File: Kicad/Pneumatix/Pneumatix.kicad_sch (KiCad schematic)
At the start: 22 parts, among them J1 Conn_01x06_Socket, J2 436500404, J3 142-0701-801, U1 E22-400T33S

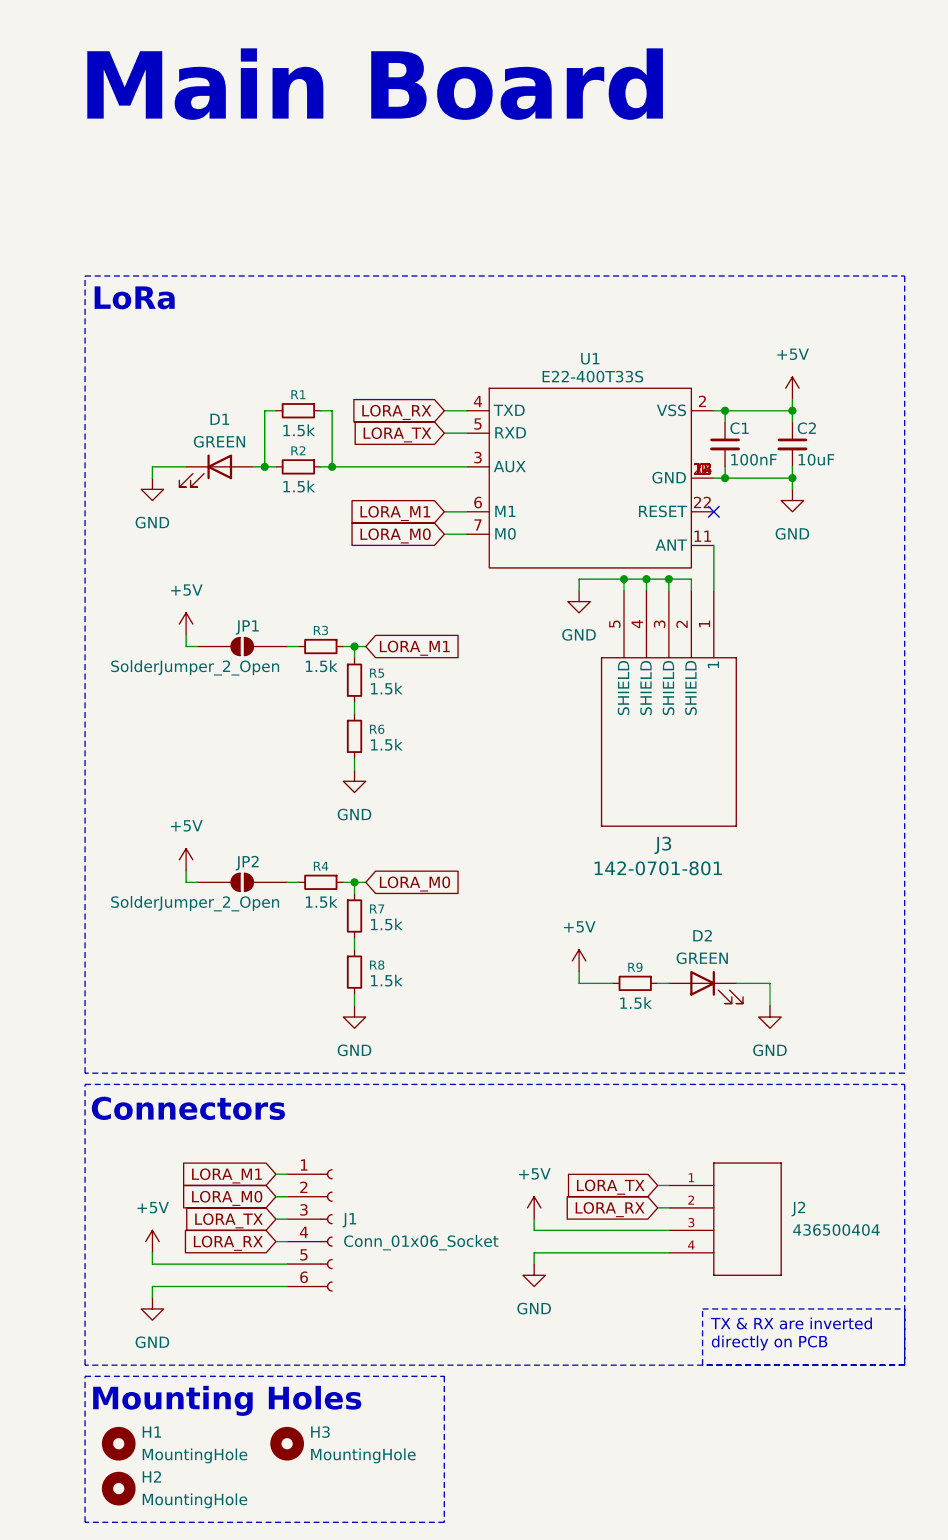
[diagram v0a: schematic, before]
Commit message: wip: pcb adjustements
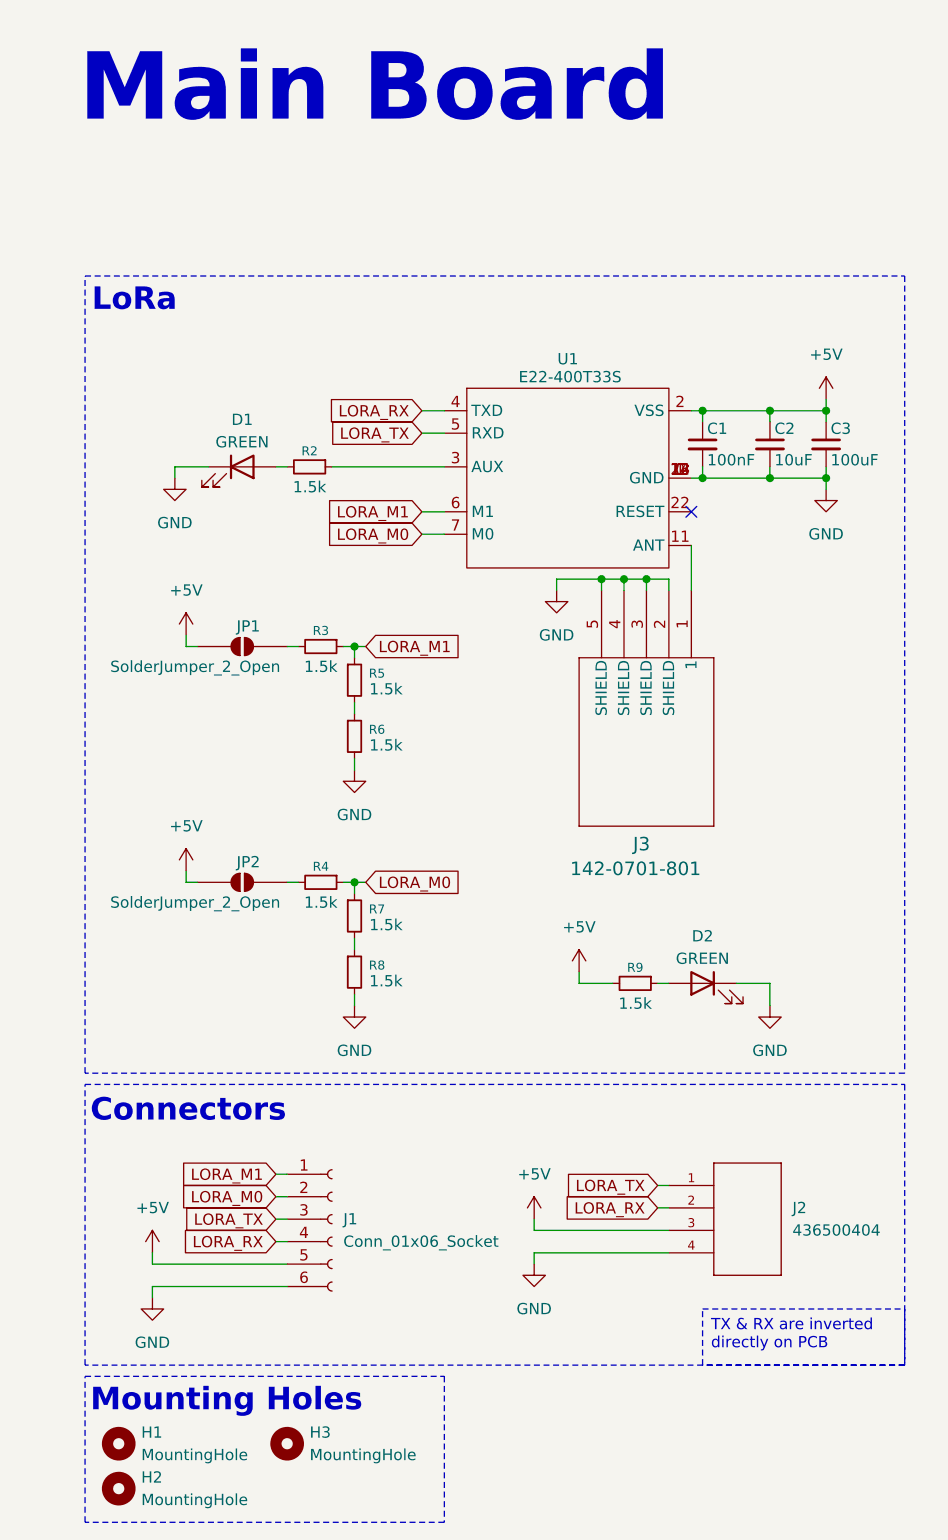
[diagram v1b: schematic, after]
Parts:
- removed R1: 1.5k, Resistor_SMD:R_0603_1608Metric, symbol Device:R_Small
- added C3: 100uF, Capacitor_SMD:C_0603_1608Metric, symbol Device:C_Small
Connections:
- net +5V: now also C3.1
- net GND: now also C3.2
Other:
- moved on the sheet: C1, C2, D1, J3, R2, U1
